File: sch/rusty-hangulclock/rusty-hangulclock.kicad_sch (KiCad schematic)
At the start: 14 parts, among them J1 Conn_OLED, J2 Conn_LEDS, J3 PWR, SW1 SW_Push, SW2 SW_Push

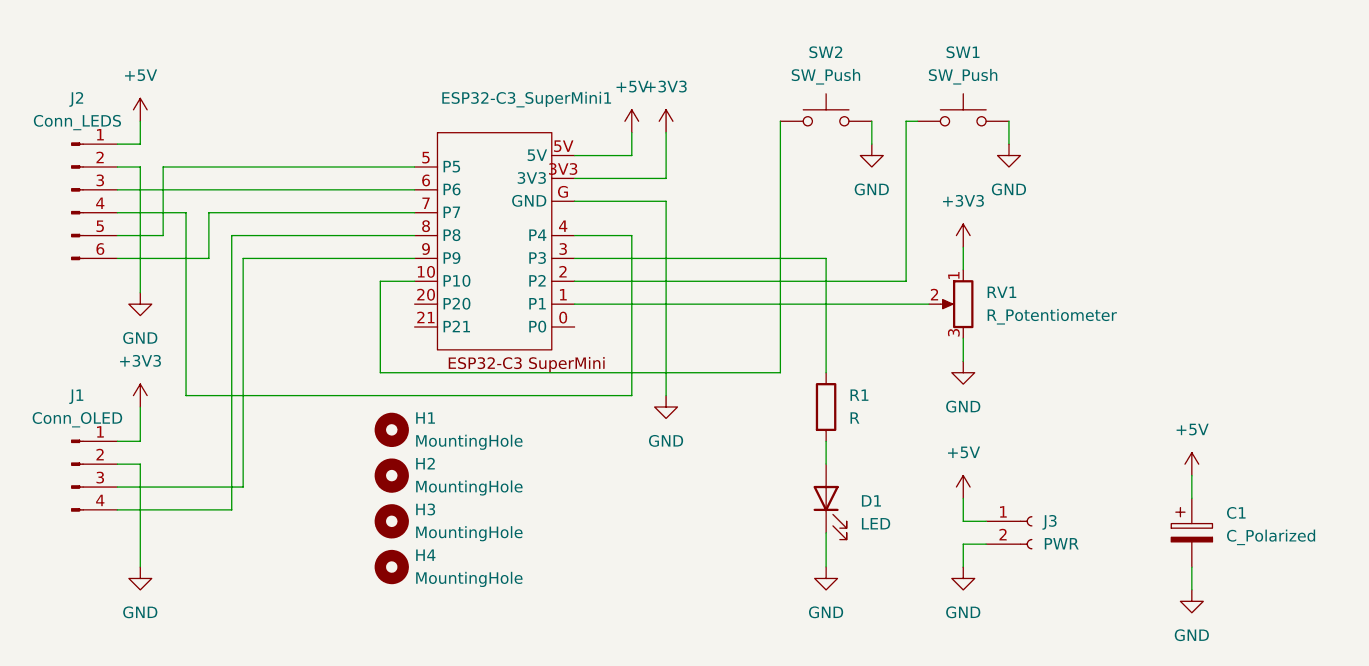
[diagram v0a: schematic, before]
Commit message: split code to files
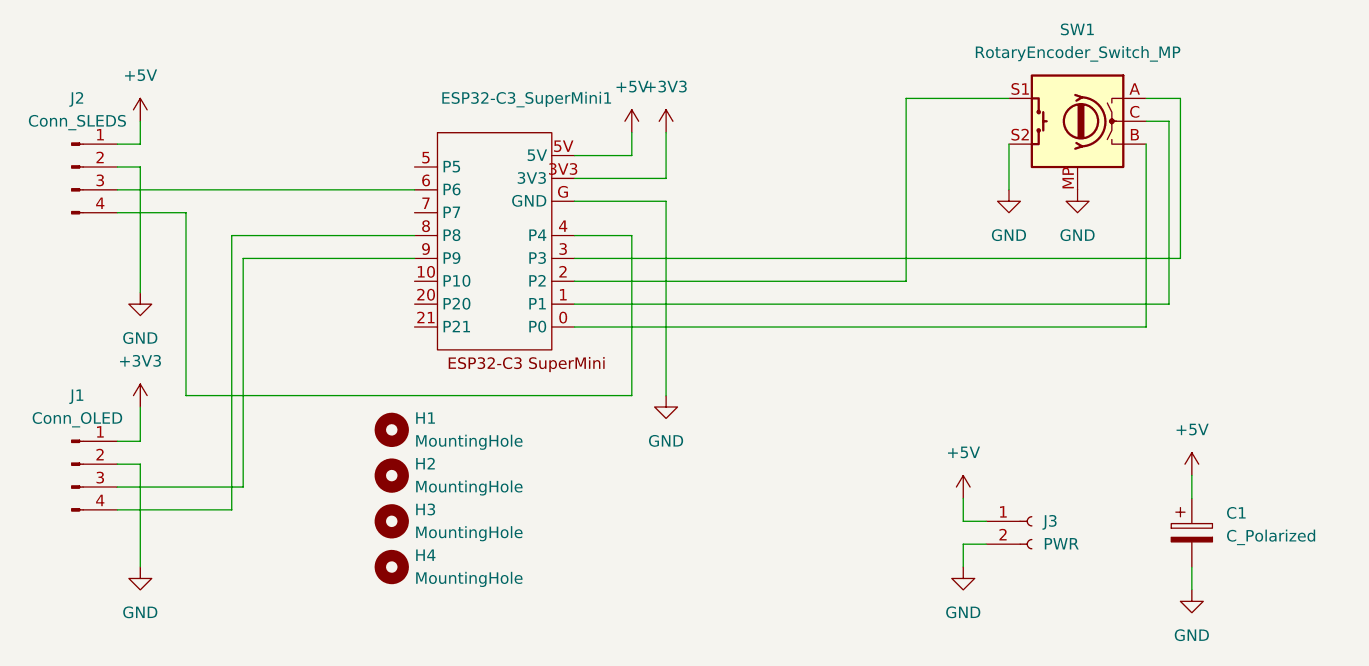
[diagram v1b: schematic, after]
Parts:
- removed D1: LED, LED_THT:LED_D3.0mm, symbol Device:LED
- removed J2: Conn_LEDS, Connector_PinHeader_2.54mm:PinHeader_1x06_P2.54mm_Horizontal, symbol Connector:Conn_01x06_Pin
- removed R1: R, Resistor_THT:R_Axial_DIN0204_L3.6mm_D1.6mm_P7.62mm_Horizontal, symbol Device:R
- removed RV1: R_Potentiometer, Potentiometer_THT:Potentiometer_ACP_CA9-V10_Vertical, symbol Device:R_Potentiometer
- removed SW1, SW2: SW_Push, Button_Switch_THT:SW_PUSH_6mm, symbol Switch:SW_Push
- added J2: Conn_SLEDS, Connector_PinHeader_2.54mm:PinHeader_1x04_P2.54mm_Horizontal, symbol Connector:Conn_01x04_Pin
- added SW1: RotaryEncoder_Switch_MP, Rotary_Encoder:RotaryEncoder_Alps_EC11E-Switch_Vertical_H20mm, symbol Device:RotaryEncoder_Switch_MP
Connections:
- net +5V: now also J2.1 (Pin_1)
- net GND: now also J2.2 (Pin_2), SW1.MP, SW1.S2
- net at ESP32-C3_SuperMini1.0 (P0): now also SW1.B
- net at ESP32-C3_SuperMini1.1 (P1): now also SW1.C
- net at ESP32-C3_SuperMini1.2 (P2): now also SW1.S1
- net at ESP32-C3_SuperMini1.3 (P3): now also SW1.A
- net at ESP32-C3_SuperMini1.4 (P4): now also J2.4 (Pin_4)
- net at ESP32-C3_SuperMini1.6 (P6): now also J2.3 (Pin_3)
